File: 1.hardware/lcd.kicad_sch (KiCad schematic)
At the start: 40 parts, among them J12 FPC_LCD_40_CONN

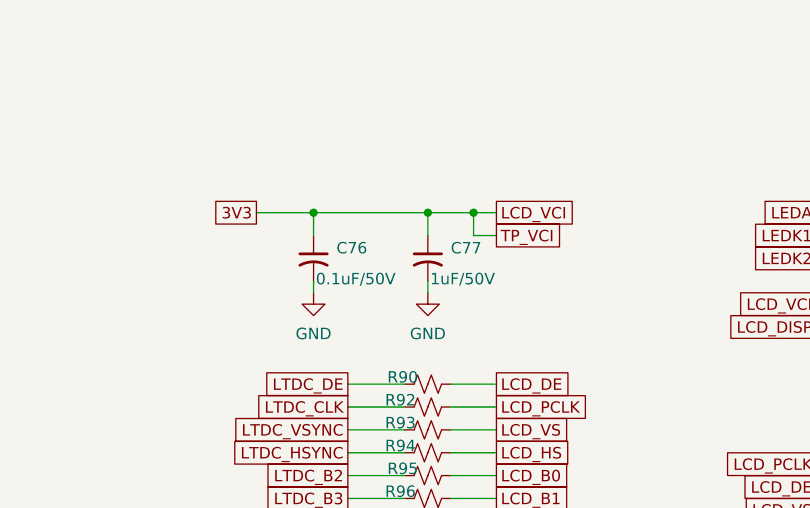
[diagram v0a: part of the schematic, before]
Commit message: 오류 일단 다 잡음
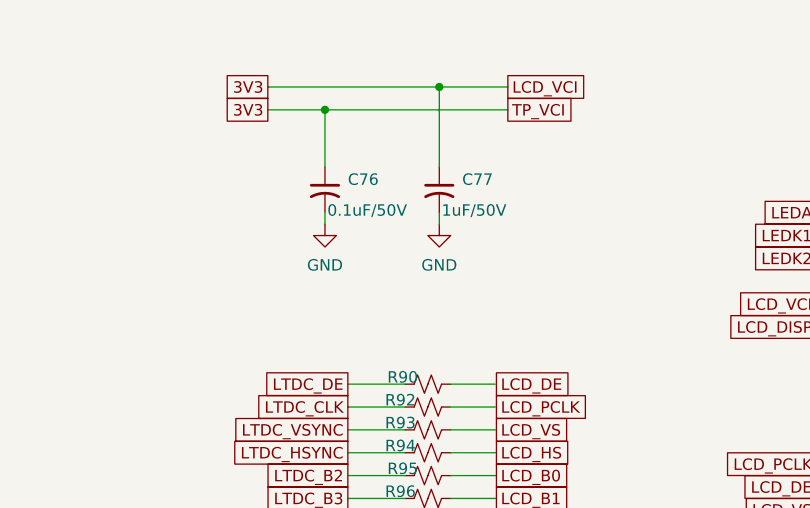
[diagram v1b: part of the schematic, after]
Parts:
- C76: footprint Capacitor_SMD:C_0603_1608Metric -> Capacitor_SMD:C_0402_1005Metric
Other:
- moved on the sheet: C76, C77
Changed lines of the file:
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@@
 	)
 	(junction
-		(at 147.32 67.31)
-		(diameter 0)
-		(color 0 0 0 0)
-	)
-	(junction
-		(at 243.84 64.77)
+		(at 245.11 53.34)
 		(diameter 0)
 		(color 0 0 0 0)
 	)
 	(junction
-		(at 261.62 64.77)
+		(at 147.32 67.31)
 		(diameter 0)
 		(color 0 0 0 0)
@@
 	)
 	(junction
-		(at 256.54 64.77)
+		(at 257.81 50.8)
 		(diameter 0)
 		(color 0 0 0 0)
@@
 	(wire
 		(pts
-			(xy 256.54 67.31) (xy 256.54 64.77)
+			(xy 257.81 59.69) (xy 257.81 50.8)
 		)
 		(stroke
@@
 	(wire
 		(pts
+			(xy 245.11 53.34) (xy 265.43 53.34)
+		)
+		(stroke
+			(width 0)
+			(type default)
+		)
+	)
+	(wire
+		(pts
 			(xy 247.65 96.52) (xy 254 96.52)
 		)
@@
 	(wire
 		(pts
-			(xy 243.84 64.77) (xy 256.54 64.77)
+			(xy 238.76 53.34) (xy 245.11 53.34)
 		)
 		(stroke
@@
 	(wire
 		(pts
-			(xy 243.84 72.39) (xy 243.84 73.66)
+			(xy 245.11 64.77) (xy 245.11 66.04)
 		)
 		(stroke
@@
 	(wire
 		(pts
-			(xy 264.16 67.31) (xy 261.62 67.31)
-		)
-		(stroke
-			(width 0)
-			(type default)
-		)
-	)
-	(wire
-		(pts
 			(xy 144.78 77.47) (xy 149.86 77.47)
 		)
@@
 	(wire
 		(pts
-			(xy 243.84 64.77) (xy 243.84 67.31)
-		)
-		(stroke
-			(width 0)
-			(type default)
-		)
-	)
-	(wire
-		(pts
 			(xy 186.69 82.55) (xy 186.69 83.82)
 		)
@@
 	(wire
 		(pts
-			(xy 261.62 64.77) (xy 264.16 64.77)
-		)
-		(stroke
-			(width 0)
-			(type default)
-		)
-	)
-	(wire
-		(pts
 			(xy 299.72 120.65) (xy 304.8 120.65)
 		)
@@
 	(wire
 		(pts
-			(xy 237.49 64.77) (xy 243.84 64.77)
+			(xy 238.76 50.8) (xy 257.81 50.8)
 		)
 		(stroke
@@
 	(wire
 		(pts
-			(xy 256.54 72.39) (xy 256.54 73.66)
-		)
-		(stroke
-			(width 0)
-			(type default)
-		)
-	)
-	(wire
-		(pts
-			(xy 261.62 67.31) (xy 261.62 64.77)
+			(xy 257.81 64.77) (xy 257.81 66.04)
 		)
 		(stroke
@@
 	(wire
 		(pts
-			(xy 256.54 64.77) (xy 261.62 64.77)
+			(xy 257.81 50.8) (xy 265.43 50.8)
 		)
 		(stroke
@@
 	(wire
 		(pts
+			(xy 245.11 53.34) (xy 245.11 59.69)
+		)
+		(stroke
+			(width 0)
+			(type default)
+		)
+	)
+	(wire
+		(pts
 			(xy 137.16 67.31) (xy 137.16 68.58)
 		)
@@
 		)
 	)
+	(global_label "3V3"
+		(shape passive)
+		(at 238.76 53.34 180)
+		(fields_autoplaced yes)
+		(effects
+			(font
+				(size 1.27 1.27)
+			)
+			(justify right)
+		)
+		(property "Intersheetrefs" "${INTERSHEET_REFS}"
+			(at 233.3785 53.34 0)
+			(effects
+				(font
+					(size 1.27 1.27)
+				)
+				(justify right)
+				(hide yes)
+			)
+		)
+	)
 	(global_label "LCD_VCI"
 		(shape passive)
@@
 	(global_label "LCD_VCI"
 		(shape passive)
-		(at 264.16 64.77 0)
+		(at 265.43 50.8 0)
 		(fields_autoplaced yes)
 		(effects
@@
 		)
 		(property "Intersheetrefs" "${INTERSHEET_REFS}"
-			(at 273.533 64.77 0)
+			(at 274.803 50.8 0)
 			(effects
 				(font
@@
 	(global_label "3V3"
 		(shape passive)
-		(at 237.49 64.77 180)
+		(at 238.76 50.8 180)
 		(fields_autoplaced yes)
 		(effects
@@
 		)
 		(property "Intersheetrefs" "${INTERSHEET_REFS}"
-			(at 232.1085 64.77 0)
+			(at 233.3785 50.8 0)
 			(effects
 				(font
@@
 	(global_label "TP_VCI"
 		(shape passive)
-		(at 264.16 67.31 0)
+		(at 265.43 53.34 0)
 		(fields_autoplaced yes)
 		(effects
@@
 		)
 		(property "Intersheetrefs" "${INTERSHEET_REFS}"
-			(at 272.2025 67.31 0)
+			(at 273.4725 53.34 0)
 			(effects
 				(font
@@
 	(symbol
 		(lib_id "power:GND")
-		(at 243.84 73.66 0)
+		(at 245.11 66.04 0)
 		(unit 1)
 		(exclude_from_sim no)
@@
 		(dnp no)
 		(property "Reference" "#PWR0104"
-			(at 243.84 80.01 0)
+			(at 245.11 72.39 0)
 			(effects
 				(font
@@
 		)
 		(property "Value" "GND"
-			(at 243.84 78.232 0)
+			(at 245.11 70.612 0)
 			(effects
 				(font
@@
 		)
 		(property "Footprint" ""
-			(at 243.84 73.66 0)
+			(at 245.11 66.04 0)
 			(effects
 				(font
@@
 		)
 		(property "Datasheet" ""
-			(at 243.84 73.66 0)
+			(at 245.11 66.04 0)
 			(effects
 				(font
@@
 		)
 		(property "Description" "Power symbol creates a global label with name \"GND\" , ground"
-			(at 243.84 73.66 0)
+			(at 245.11 66.04 0)
 			(effects
 				(font
@@
 	(symbol
 		(lib_id "Device:C_Small_US")
-		(at 243.84 69.85 0)
+		(at 245.11 62.23 0)
 		(unit 1)
 		(exclude_from_sim no)
@@
 		(dnp no)
 		(property "Reference" "C76"
-			(at 246.38 68.7069 0)
+			(at 247.65 61.0869 0)
 			(effects
 				(font
@@
 		)
 		(property "Value" "0.1uF/50V"
-			(at 244.094 72.136 0)
+			(at 245.364 64.516 0)
 			(effects
 				(font
@@
 			)
 		)
-		(property "Footprint" "Capacitor_SMD:C_0603_1608Metric"
-			(at 243.84 69.85 0)
+		(property "Footprint" "Capacitor_SMD:C_0402_1005Metric"
+			(at 245.11 62.23 0)
 			(effects
 				(font
@@
 		)
 		(property "Datasheet" ""
-			(at 243.84 69.85 0)
+			(at 245.11 62.23 0)
 			(effects
 				(font
@@
 		)
 		(property "Description" "capacitor, small US symbol"
-			(at 243.84 69.85 0)
+			(at 245.11 62.23 0)
 			(effects
 				(font
@@
 	(symbol
 		(lib_id "power:GND")
-		(at 256.54 73.66 0)
+		(at 257.81 66.04 0)
 		(unit 1)
 		(exclude_from_sim no)
@@
 		(dnp no)
 		(property "Reference" "#PWR0105"
-			(at 256.54 80.01 0)
+			(at 257.81 72.39 0)
 			(effects
 				(font
@@
 		)
 		(property "Value" "GND"
-			(at 256.54 78.232 0)
+			(at 257.81 70.612 0)
 			(effects
 				(font
@@
 		)
 		(property "Footprint" ""
-			(at 256.54 73.66 0)
+			(at 257.81 66.04 0)
 			(effects
 				(font
@@
 		)
 		(property "Datasheet" ""
-			(at 256.54 73.66 0)
+			(at 257.81 66.04 0)
 			(effects
 				(font
@@
 		)
 		(property "Description" "Power symbol creates a global label with name \"GND\" , ground"
-			(at 256.54 73.66 0)
+			(at 257.81 66.04 0)
 			(effects
 				(font
@@
 	(symbol
 		(lib_id "Device:C_Small_US")
-		(at 256.54 69.85 0)
+		(at 257.81 62.23 0)
 		(unit 1)
 		(exclude_from_sim no)
@@
 		(dnp no)
 		(property "Reference" "C77"
-			(at 259.08 68.7069 0)
+			(at 260.35 61.0869 0)
 			(effects
 				(font
@@
 		)
 		(property "Value" "1uF/50V"
-			(at 256.794 72.136 0)
+			(at 258.064 64.516 0)
 			(effects
 				(font
@@
 		)
 		(property "Footprint" "Capacitor_SMD:C_0603_1608Metric"
-			(at 256.54 69.85 0)
+			(at 257.81 62.23 0)
 			(effects
 				(font
@@
 		)
 		(property "Datasheet" ""
-			(at 256.54 69.85 0)
+			(at 257.81 62.23 0)
 			(effects
 				(font
@@
 		)
 		(property "Description" "capacitor, small US symbol"
-			(at 256.54 69.85 0)
+			(at 257.81 62.23 0)
 			(effects
 				(font
